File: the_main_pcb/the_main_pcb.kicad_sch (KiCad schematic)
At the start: 1 part

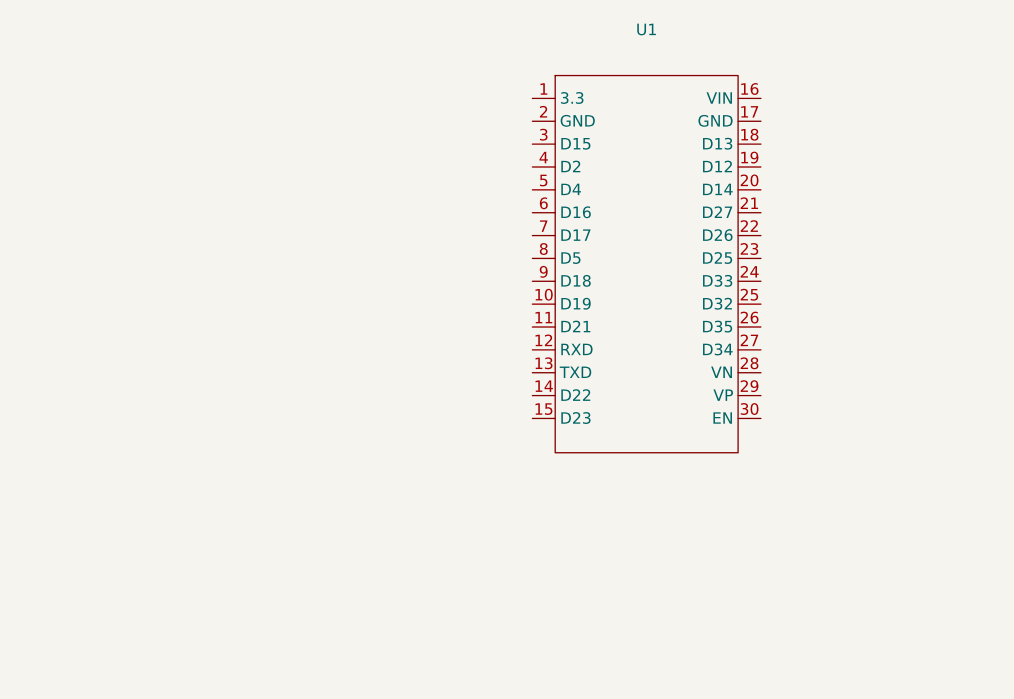
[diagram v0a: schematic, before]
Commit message: worked more on the pcb
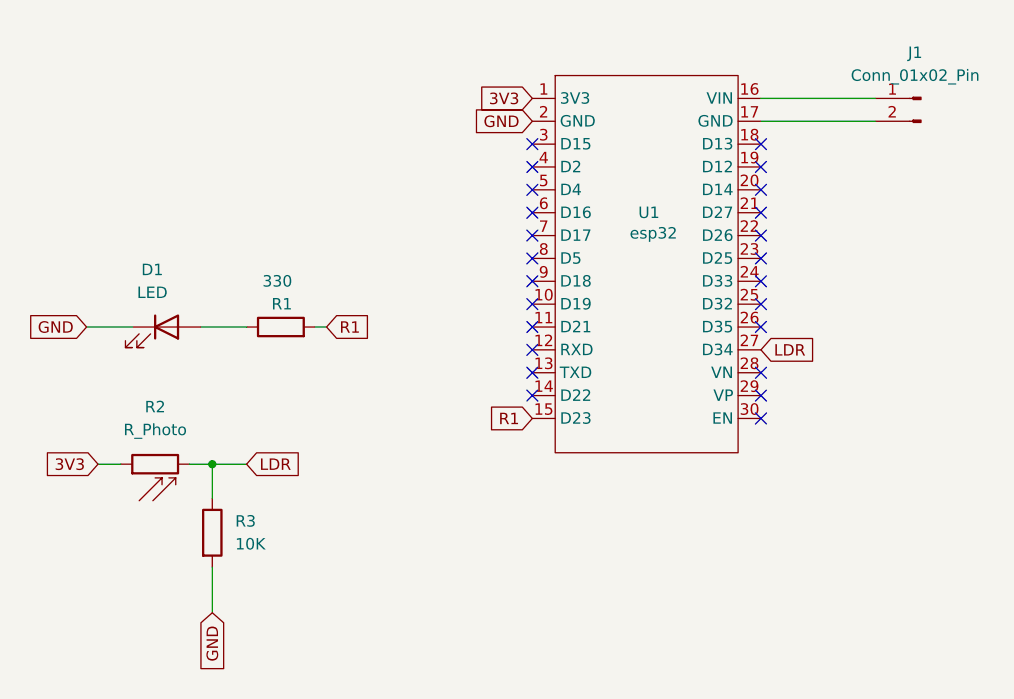
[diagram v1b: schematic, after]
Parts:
- added D1: LED, LED_THT:LED_D1.8mm_W3.3mm_H2.4mm, symbol Device:LED
- added J1: Conn_01x02_Pin, Connector_PinHeader_2.54mm:PinHeader_1x02_P2.54mm_Vertical, symbol Connector:Conn_01x02_Pin
- added R1: 330, Resistor_THT:R_Axial_DIN0309_L9.0mm_D3.2mm_P12.70mm_Horizontal, symbol Device:R
- added R2: R_Photo, LED_THT:LED_D1.8mm_W3.3mm_H2.4mm, symbol Device:R_Photo
- added R3: 10K, Resistor_THT:R_Axial_DIN0309_L9.0mm_D3.2mm_P12.70mm_Horizontal, symbol Device:R
- U1: value ~ -> esp32
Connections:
- net 3V3: now reaches U1.1 (3V3)
- net 3V3: now also R2.1
- net R1: now reaches U1.15 (D23)
- net R1: now also R1.2
- net at U1.16 (VIN): now also J1.1 (Pin_1)
- net at U1.17 (GND): now also J1.2 (Pin_2)
- net GND: now reaches U1.2 (GND)
- net GND: now also D1.1 (K), R3.2
- net LDR: now reaches U1.27 (D34)
- net LDR: now also R2.2, R3.1
- new net: D1.2 (A), R1.1
- no-connect marks 0 -> 24
